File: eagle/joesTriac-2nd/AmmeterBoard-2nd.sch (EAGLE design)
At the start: 41 parts, among them IC10 LM317MB, IC12 LM337, IC13 TLC251P, IC14 TLC251P, IC15 TLC251P, IC6 TLC251P, IC7 ACS758ECB-200B-PFF-T, IC8 X9C104P, X1 1, X2 2, X6 1751264

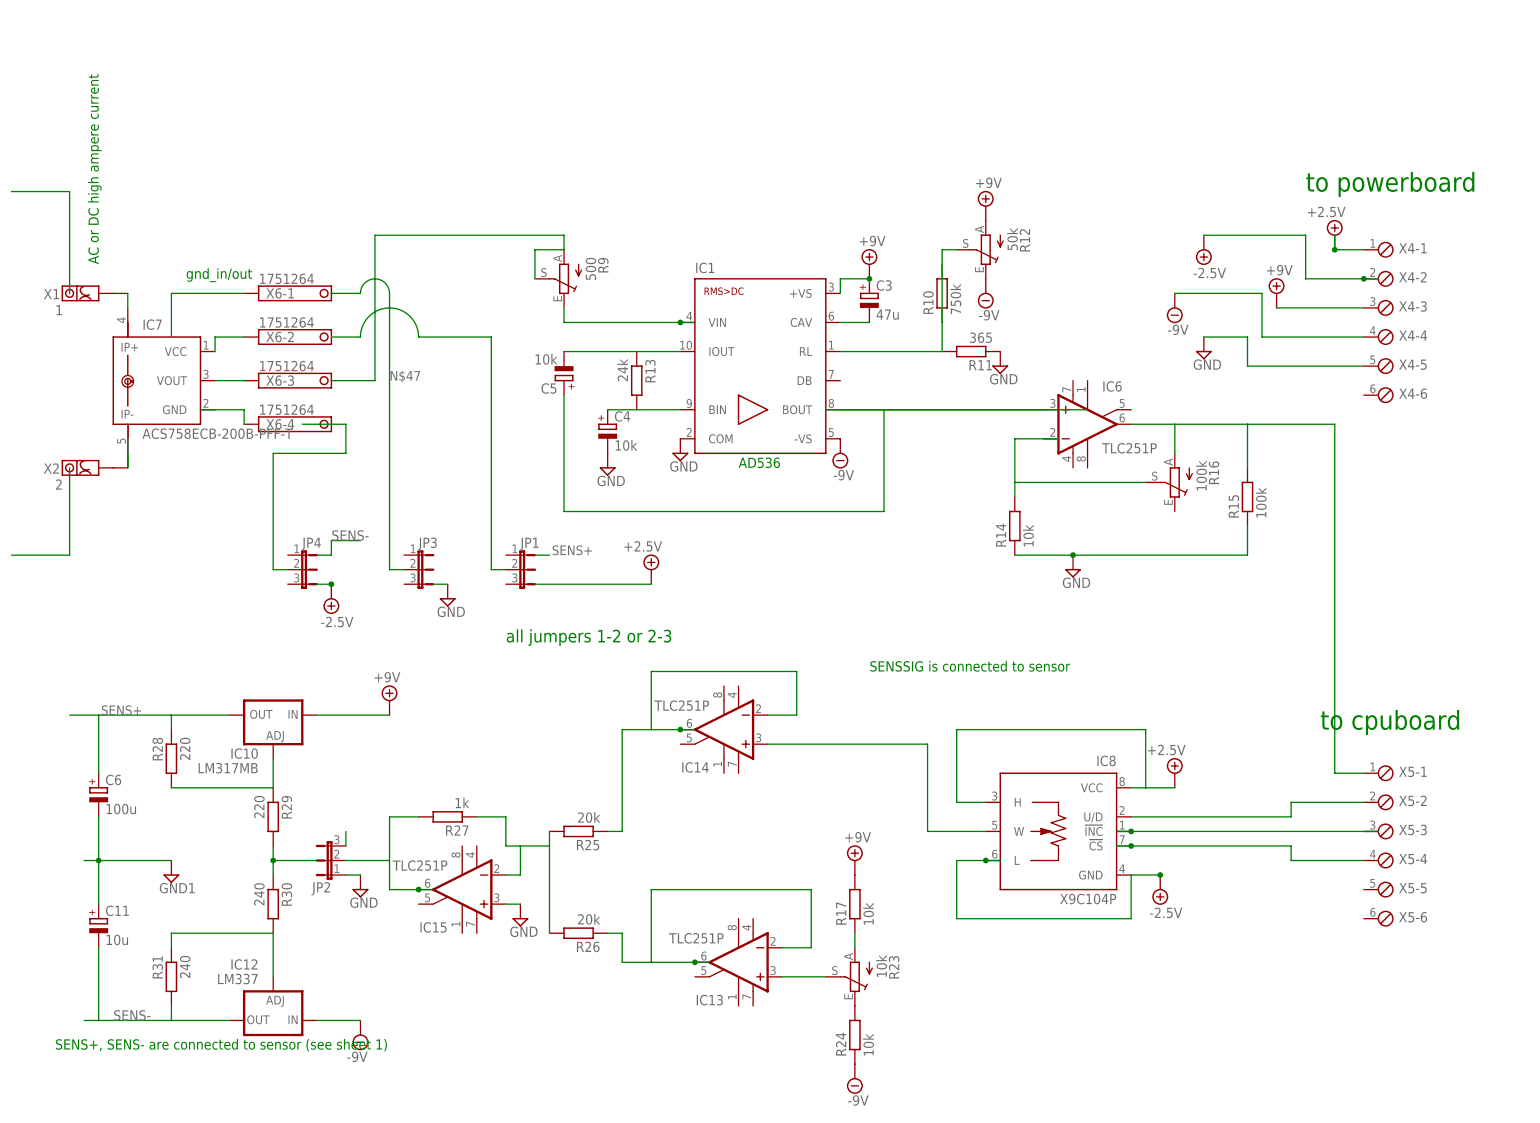
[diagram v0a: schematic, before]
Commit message: reg save
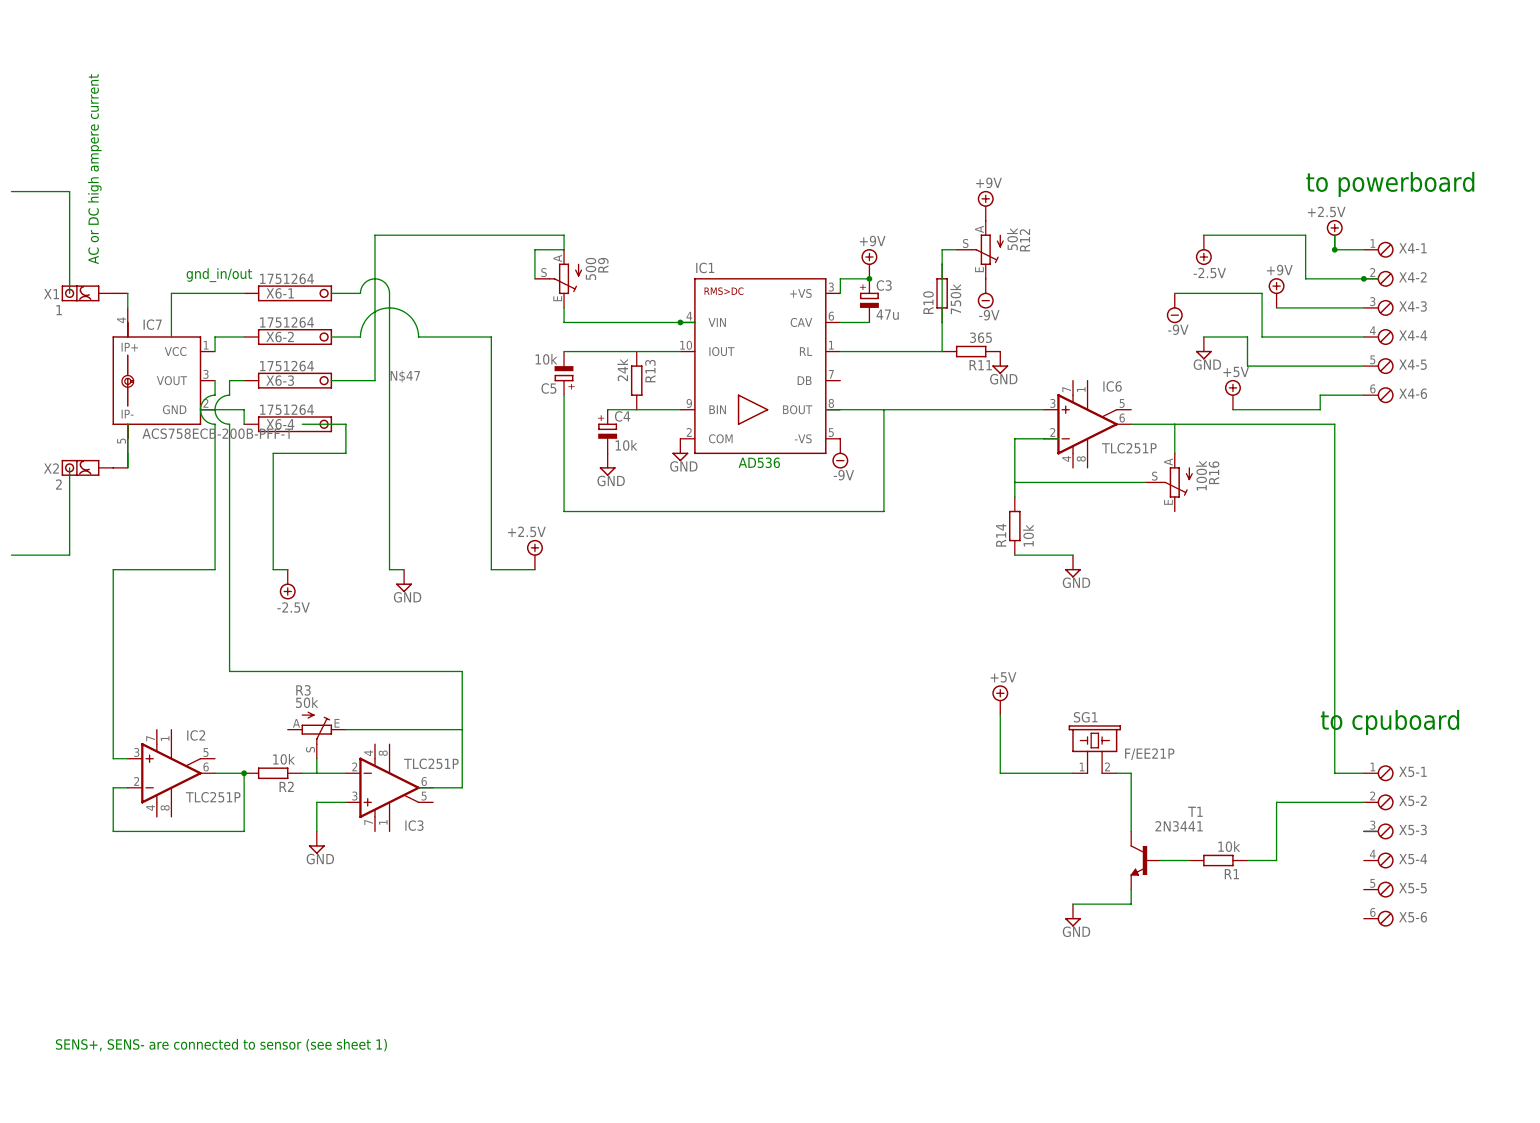
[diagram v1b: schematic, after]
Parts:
- removed C11: 10u, resistor:CPOL-EUE5-10.5
- removed C6: 100u, resistor:CPOL-EUE5-10.5
- removed IC10: LM317MB, v-reg:LM317MB
- removed IC12: LM337, v-reg:LM337TL
- removed IC13, IC14, IC15: TLC251P, linear:TLC251P
- removed IC8: X9C104P, pot-xicor:X9C102P
- removed JP1, JP2, JP3, JP4: (no value), jumper:JP2E
- removed R15: 100k, resistor:R-EU_0207/10
- removed R17, R24: 10k, resistor:R-EU_0207/10
- removed R23: 10k, pot:TRIM_EU-B90P
- removed R25, R26: 20k, resistor:R-EU_0207/10
- removed R27: 1k, resistor:R-EU_0207/10
- removed R28, R29: 220, resistor:R-EU_0207/10
- removed R30, R31: 240, resistor:R-EU_0207/10
- added IC2, IC3: TLC251P, linear:TLC251P
- added R1, R2: 10k, resistor:R-EU_0207/10
- added R3: 50k, pot:TRIM_EU-B90P
- added SG1: F/EE21P, buzzer:F/EE21P
- added T1: 2N3441, transistor:2N3441
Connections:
- removed net GND1: C11.+, C6.-
- removed net N$15: JP3.2
- removed net N$24: IC1.BOUT
- removed net N$32: IC8.!CS, X5-4.1
- removed net N$33: IC13.+IN, R23.S
- removed net N$34: R17.1, R23.A
- removed net N$35: R23.E, R24.2
- removed net N$36: IC13.-IN, IC13.OUT, R26.1
- removed net N$37: IC14.+IN, IC8.W
- removed net N$38: IC14.-IN, IC14.OUT, R25.1
- removed net N$39: R29.2, R30.1
- removed net N$40: IC15.OUT, JP2.2, R27.2
- removed net N$41: IC15.-IN, R25.2, R26.2, R27.1
- removed net N$42: IC10.ADJ, R28.2, R29.1
- removed net SENS+: C6.+, IC10.OUT, R28.1
- removed net SENS-: C11.-, IC12.ADJ, IC12.OUT, R30.2, R31.1, R31.2
- new net +5V: SG1.1, X4-6.1
- new net N$11: IC2.-IN, IC2.OUT, R2.2
- new net N$7: SG1.2, T1.C
- net +4.1V: no longer IC8.H, IC8.VCC
- net +9V: no longer IC10.IN, R17.2
- net -4.1V: no longer IC8.GND, IC8.L
- net -9V: no longer IC12.IN, R24.1
- net GND: now also IC3.+IN, T1.E; no longer IC15.+IN, JP2.1, R15.1
- net N$1: now also R3.E, X6-3.K; no longer JP2.3
- net N$10: now also R1.1; no longer IC8.U/D
- net N$13: now also IC3.-IN, R2.1, R3.S; no longer JP4.2
- net N$26: no longer R15.2
- net N$31: no longer IC8.!INC
- net N$5: now also IC2.+IN; no longer X6-3.K
- net N$9: now also R1.2, T1.B; no longer JP1.2
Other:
- note removed: "SENSSIG is connected to sensor"
- note removed: "all jumpers 1-2 or 2-3"

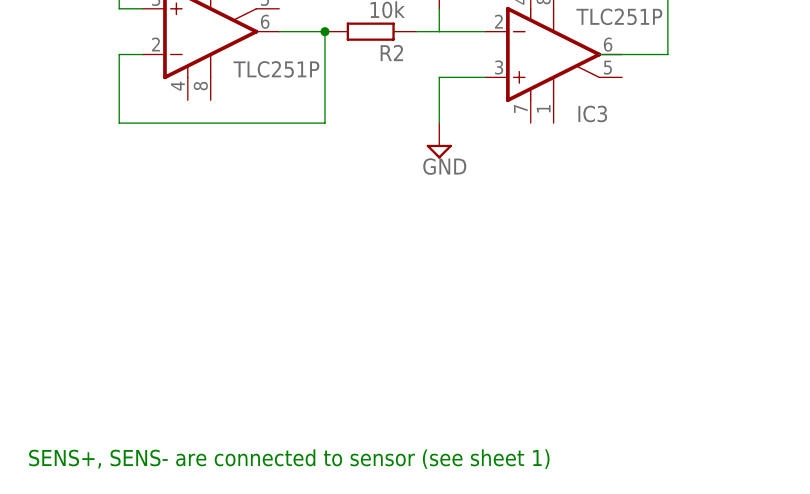
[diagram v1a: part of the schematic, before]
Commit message: reg save
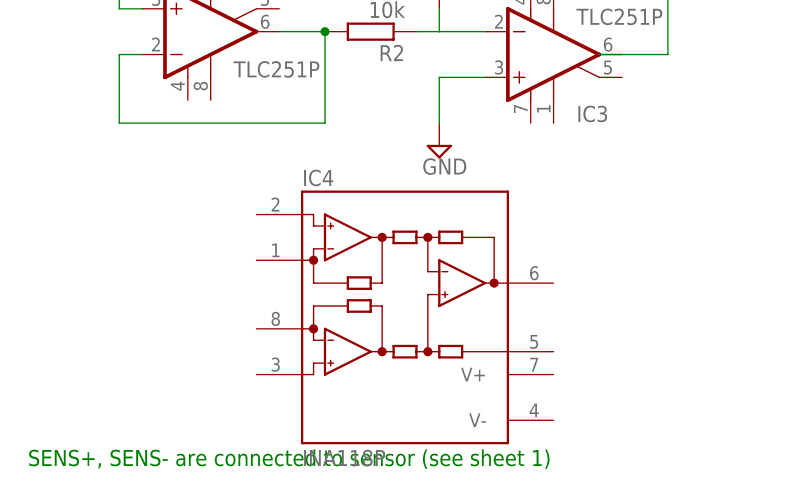
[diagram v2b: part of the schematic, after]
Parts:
- added IC4: INA118P, burr-brown:INA118P
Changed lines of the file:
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@@
 <part name="R3" library="pot" deviceset="TRIM_EU-" device="B90P" value="50k"/>
 <part name="SUPPLY20" library="supply2" deviceset="GND" device=""/>
+<part name="IC4" library="burr-brown" deviceset="INA118" device="P"/>
 </parts>
 <sheets>
@@
 <instance part="R3" gate="1" x="10.16" y="22.86" rot="R270"/>
 <instance part="SUPPLY20" gate="GND" x="10.16" y="2.54"/>
+<instance part="IC4" gate="G$1" x="7.62" y="-17.78"/>
 </instances>
 <busses>
